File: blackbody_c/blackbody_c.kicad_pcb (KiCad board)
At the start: 2 copper layers, 31.4 x 24.8 mm, 32 parts, among them IC1 MCP96L00T-E_MX, J2 Conn_01x02, U2 LTC4316IMS-PBF

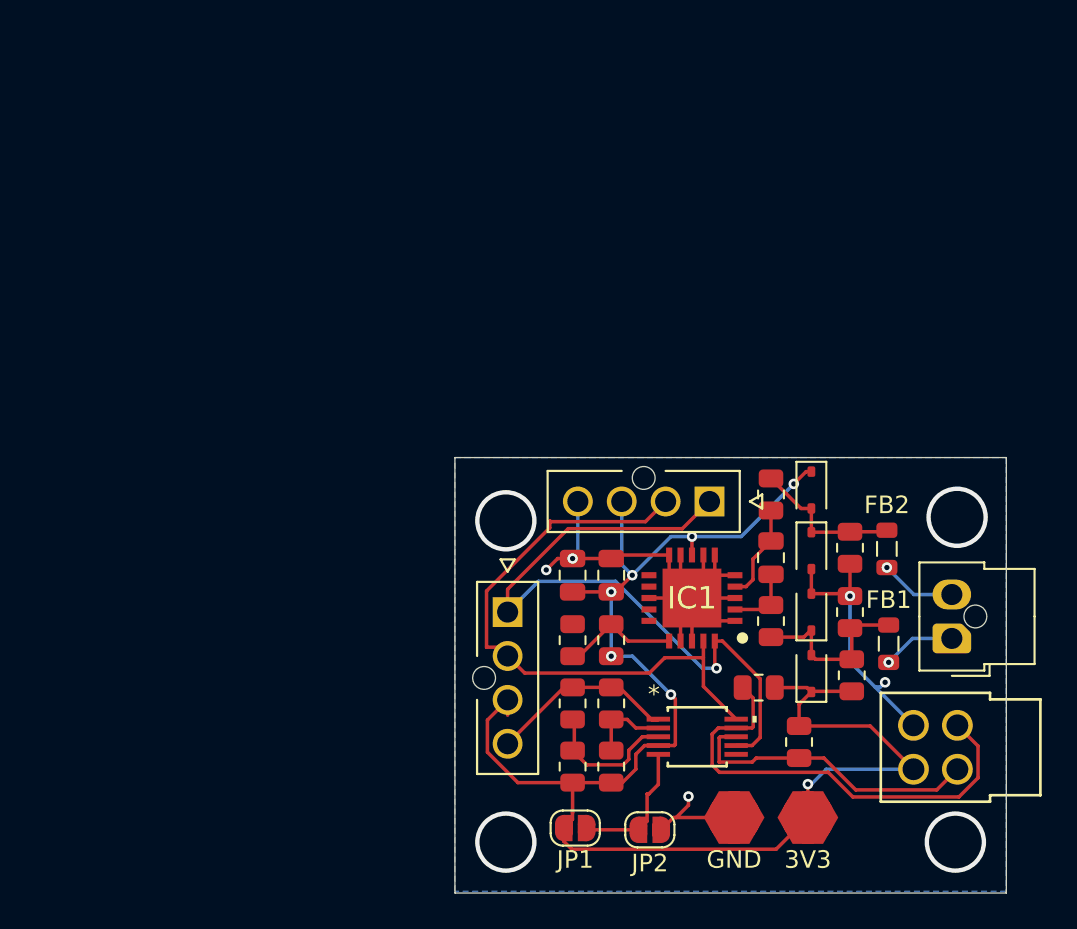
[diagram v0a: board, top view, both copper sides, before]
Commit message: layout edits
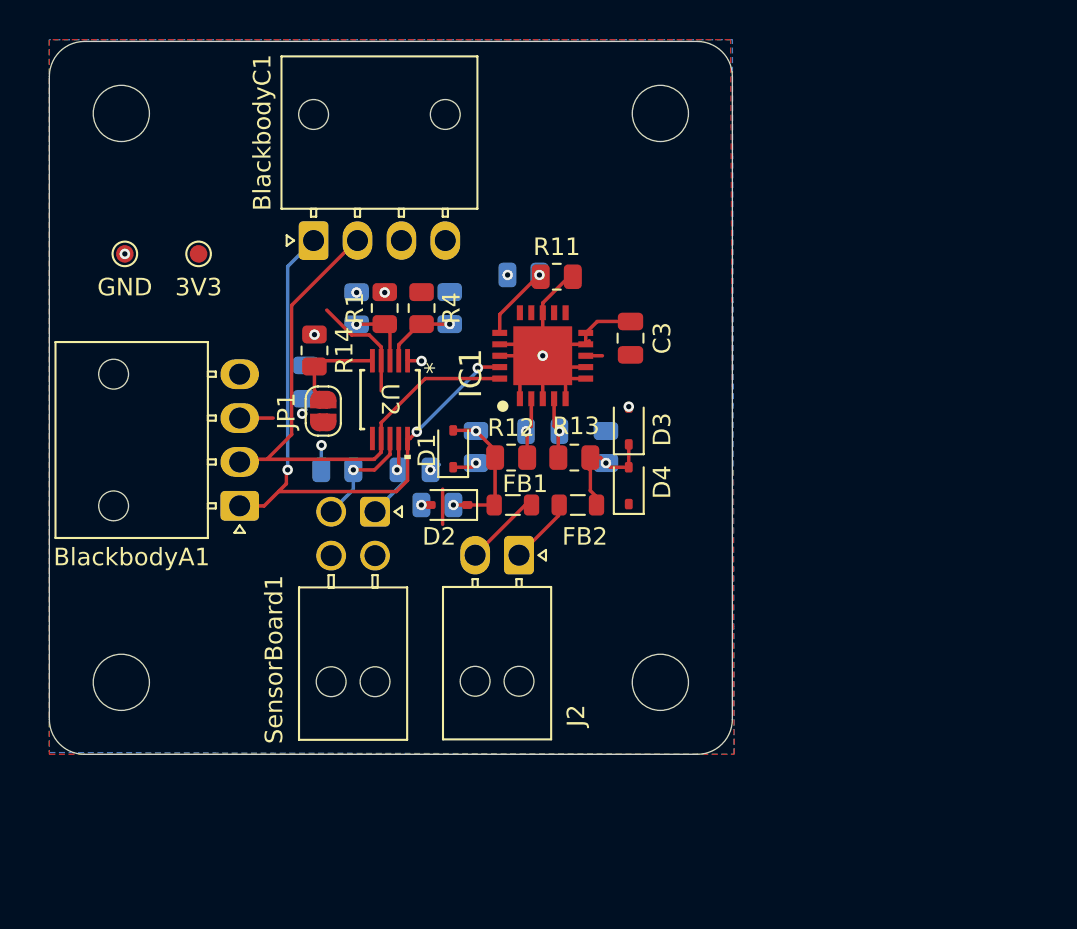
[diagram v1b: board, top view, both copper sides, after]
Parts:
- removed the GND at (92.9, 98.0)
- removed JP2: SolderJumper_2_Open, Jumper:SolderJumper-2_P1.3mm_Open_RoundedPad1.0x1.5mm
- removed irradiance: Conn_01x04, Blackbodies:CONN_SD-105310-100_04_MOL
- added GND: TestPoint, TestPoint:TestPoint_Pad_D1.0mm, F.Cu at (58.2, 65.9)
- added H1: MountingHole, MountingHole:MountingHole_3.2mm_M3, F.Cu at (58.0, 90.3)
- added H2: MountingHole, MountingHole:MountingHole_3.2mm_M3, F.Cu at (88.7, 57.9)
- added H3: MountingHole, MountingHole:MountingHole_3.2mm_M3, F.Cu at (58.0, 57.9)
- added H4: MountingHole, MountingHole:MountingHole_3.2mm_M3, F.Cu at (88.7, 90.3)
- added R14: 10k, Resistor_SMD:R_0805_2012Metric, F.Cu at (69.0, 71.4)
- added SensorBoard1: Conn_01x04, Connector_Molex:Molex_Nano-Fit_105314-xx04_2x02_P2.50mm_Horizontal, F.Cu at (72.5, 80.6)
- 3V3: footprint UTSVT_Special:TestPoint_HEX_3mmID -> TestPoint:TestPoint_Pad_D1.0mm
- BlackbodyA1, BlackbodyC1: footprint Blackbodies:MOLEX_1053091104 -> Connector_Molex:Molex_Nano-Fit_105313-xx04_1x04_P2.50mm_Horizontal
- C2, C4, R10, R2, R3, R5, R6, R7, R8, R9: moved to B.Cu
- J2: footprint Connector_Molex:Molex_Nano-Fit_105309-xx02_1x02_P2.50mm_Vertical -> Connector_Molex:Molex_Nano-Fit_105313-xx02_1x02_P2.50mm_Horizontal
- moved 3V3 47.3 mm to (62.4, 65.9), turned to 0 degrees
- moved R5 30.5 mm to (70.3, 78.2), turned to 0 degrees
- moved R3 28.9 mm to (71.4, 69.0), turned to 90 degrees
- moved R4 28.3 mm to (75.1, 69.0), turned to 90 degrees
- moved JP1 27.7 mm to (69.5, 74.8), turned to -90 degrees
- moved BlackbodyA1 26.8 mm to (64.7, 80.2)
- moved U2 26.0 mm to (73.3, 74.2), turned to -90 degrees
- moved J2 25.1 mm to (80.7, 83.1), turned to -90 degrees
- moved R9 25.0 mm to (78.2, 76.9)
- moved R1 24.9 mm to (73.0, 69.0)
- moved R2 24.3 mm to (76.7, 69.0)
- moved R8 24.3 mm to (76.0, 80.2), turned to 0 degrees
- moved D1 24.1 mm to (76.9, 77.0)
- moved BlackbodyC1 23.9 mm to (69.0, 65.1), turned to 90 degrees
- moved R6 23.2 mm to (74.7, 78.2)
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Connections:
- BlackbodyA1 pad 1: /SDA -> /SCL
- BlackbodyA1 pad 2: /SCL -> /SDA
- BlackbodyC1 pad 1: /SDA -> /SCL
- BlackbodyC1 pad 2: /SCL -> /SDA
- J2 pad 1: Net-(J2-Pin_1) -> Net-(J2-Pin_2)
- J2 pad 2: Net-(J2-Pin_2) -> Net-(J2-Pin_1)
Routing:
- net +3V3: track 91.3 -> 15.1 mm, vias 7 -> 6
- net GND: track 68.1 -> 30.7 mm, vias 5 -> 7
- net /irradiance/SCL_board: track 26.6 -> 5.85 mm, vias 0 -> 1
- net /irradiance/SDA_board: track 17.3 -> 6.27 mm, vias 0 -> 1
- net /SDA: track 39.5 -> 32.7 mm, vias 1 -> 0
- net Net-(U2-XORL): track 8.08 -> 3.81 mm, vias 0 -> 1
- net Net-(IC1-ADDR): track 6.65 -> 4.41 mm, vias 0 -> 1
- net Net-(JP1-A): track 7.82 -> 5.60 mm
- net Net-(IC1-VIN-): track 5.55 -> 3.50 mm, vias 0 -> 1
- net Net-(D1-A): track 10.3 -> 8.32 mm, vias 0 -> 2
- net Net-(D3-K): track 8.71 -> 6.74 mm, vias 0 -> 1
- net Net-(J2-Pin_2): track 4.34 -> 3.79 mm, vias 1 -> 0
- net Net-(IC1-VIN+): track 3.90 -> 3.50 mm, vias 0 -> 1
- net /SCL: track 34.3 -> 34.7 mm, vias 0 -> 3
- net Net-(U2-XORH): track 4.66 -> 4.31 mm, vias 0 -> 1
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- added copper zone on F.Cu, net +3V3
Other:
- board size 31.4 x 24.8 mm -> 38.9 x 40.6 mm
